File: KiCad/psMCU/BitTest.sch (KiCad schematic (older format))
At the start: 40 parts

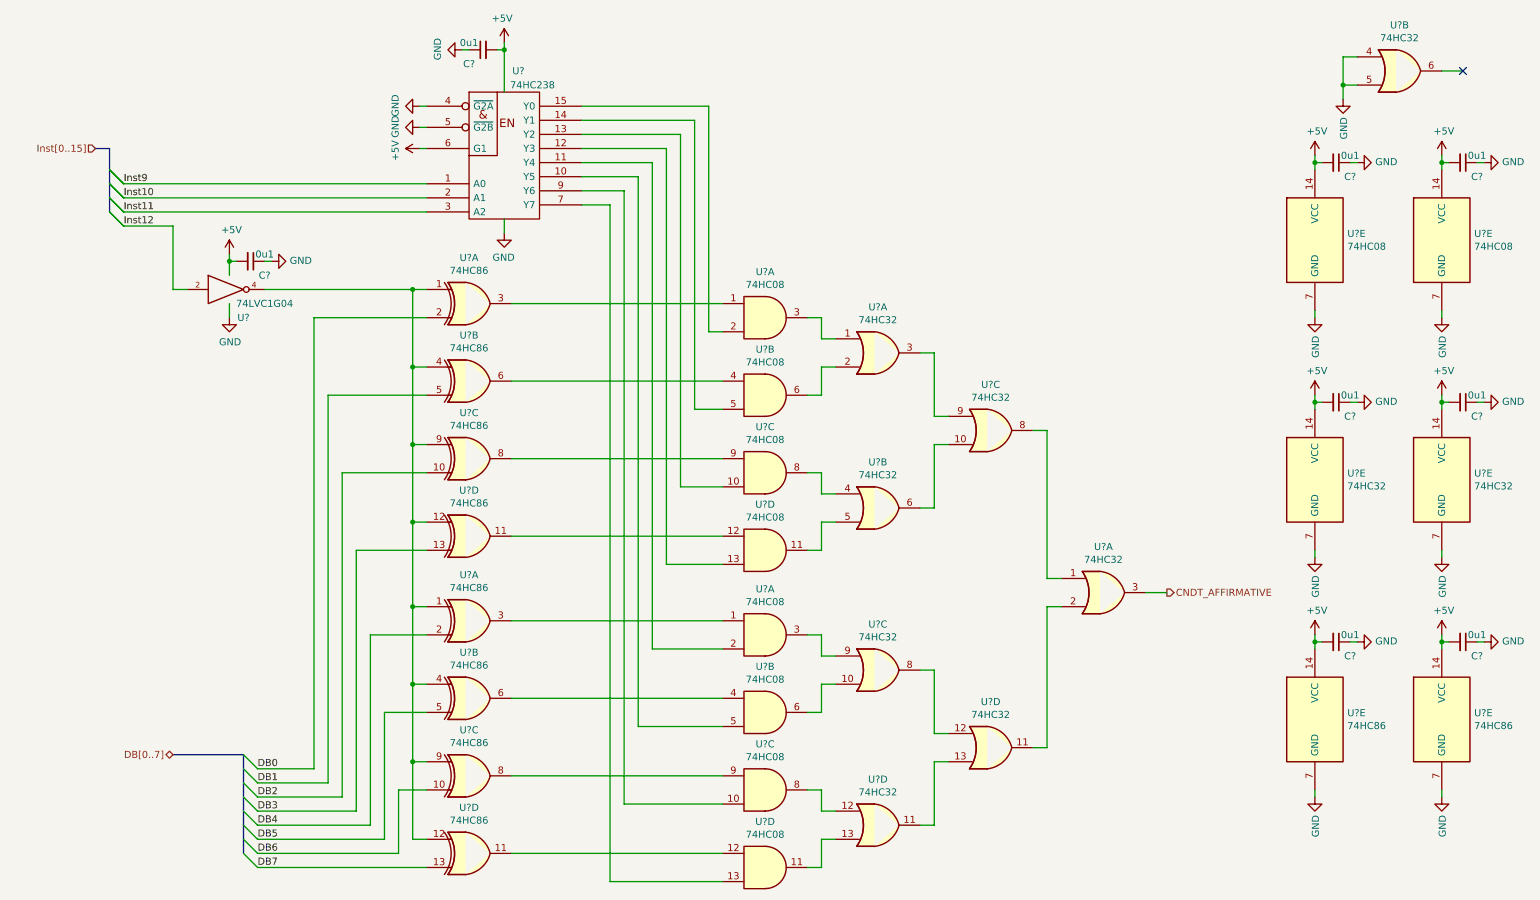
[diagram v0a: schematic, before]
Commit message: First Schematic Draft done.
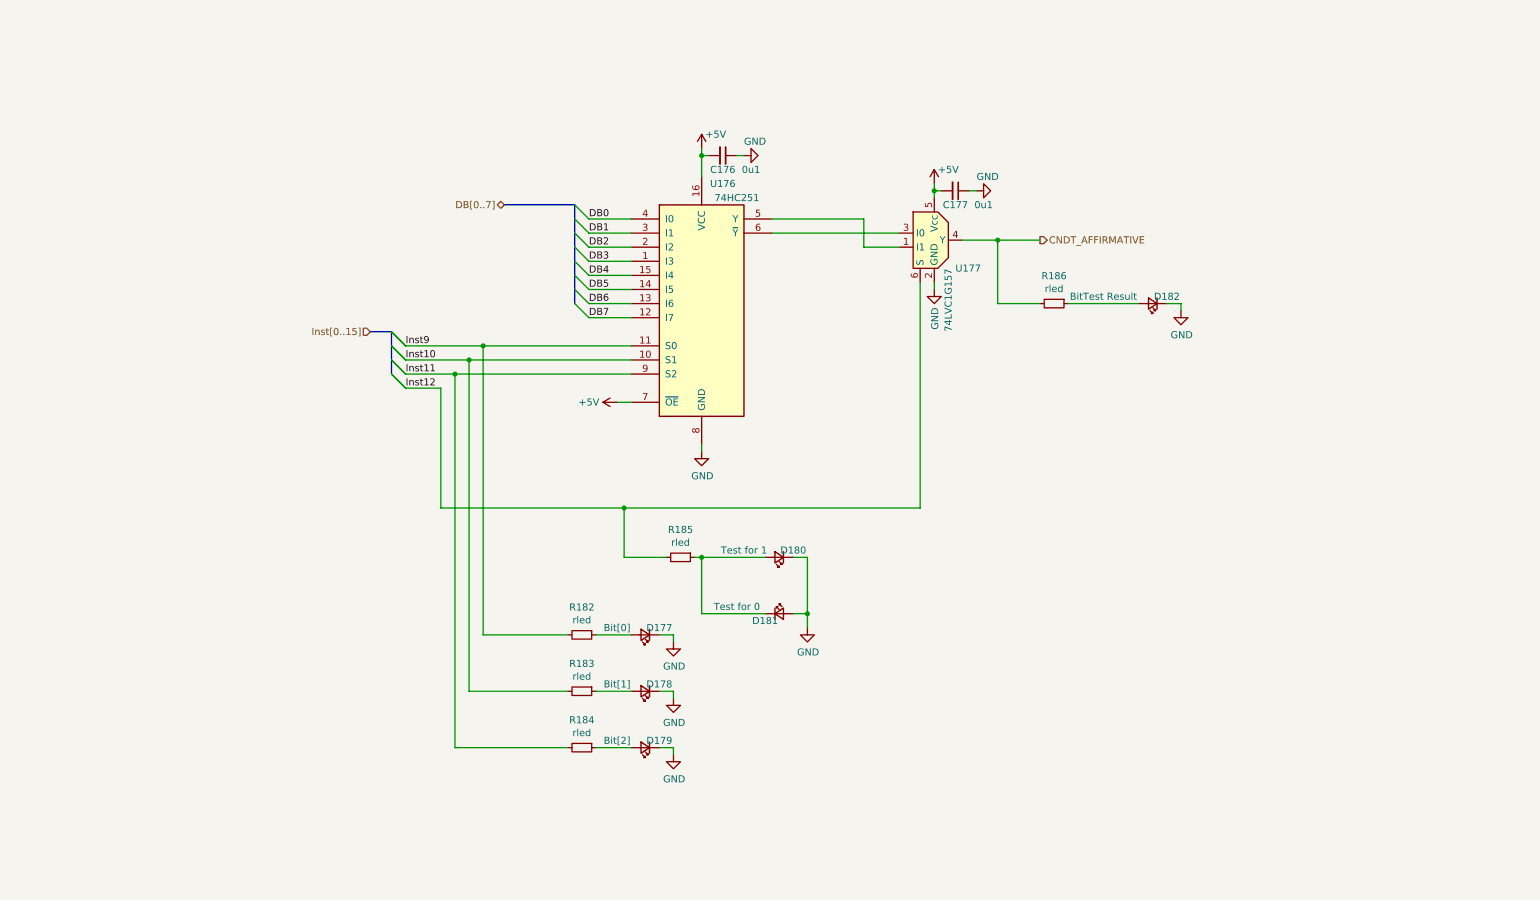
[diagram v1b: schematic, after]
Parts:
- removed C? (x8): 0u1, Capacitor_SMD:C_0603_1608Metric, symbol Device:C_Small
- removed U?: 74HC238, symbol 74xx_IEEE:74HC238
- removed U? (x10): 74HC08, symbol 74xx:74LS08
- removed U? (x10): 74HC32, symbol 74xx:74LS32
- removed U? (x10): 74HC86, symbol 74xx:74HC86
- removed U?: 74LVC1G04, Package_TO_SOT_SMD:SOT-353_SC-70-5, symbol 74xGxx:74LVC1G04
- added C176, C177: 0u1, NoRef_Footprints:C_0603_1608Metric_NoRef, symbol Device:C_Small
- added D177: Bit[0], NoRef_Footprints:D_0603_1608Metric_NoRef, symbol Device:LED_Small
- added D178: Bit[1], NoRef_Footprints:D_0603_1608Metric_NoRef, symbol Device:LED_Small
- added D179: Bit[2], NoRef_Footprints:D_0603_1608Metric_NoRef, symbol Device:LED_Small
- added D180: Test for 1, NoRef_Footprints:D_0603_1608Metric_NoRef, symbol Device:LED_Small
- added D181: Test for 0, NoRef_Footprints:D_0603_1608Metric_NoRef, symbol Device:LED_Small
- added D182: BitTest Result, NoRef_Footprints:D_0603_1608Metric_NoRef, symbol Device:LED_Small
- added R182, R183, R184, R185, R186: rled, NoRef_Footprints:R_0603_1608Metric, symbol Device:R_Small
- added U176: 74HC251, symbol 74xx:74LS251
- added U177: 74LVC1G157, Package_TO_SOT_SMD:SOT-363_SC-70-6, symbol 74LVC1G157:74LVC1G157
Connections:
- net +5V: now also C176.2, C177.2, U176.16 (VCC), U176.7 (~OE), U177.5 (Vcc)
- net CNDT_AFFIRMATIVE: now also R186.2, U177.4 (Y)
- net DB0: now also U176.4 (I0)
- net DB1: now also U176.3 (I1)
- net DB2: now also U176.2 (I2)
- net DB3: now also U176.1 (I3)
- net DB4: now also U176.15 (I4)
- net DB5: now also U176.14 (I5)
- net DB6: now also U176.13 (I6)
- net DB7: now also U176.12 (I7)
- net GND: now also C176.1, C177.1, D177.1 (K), D178.1 (K), D179.1 (K), D180.1 (K), D181.2 (A), D182.1 (K), U176.8 (GND), U177.2 (GND)
- net Inst10: now also R183.2, U176.10 (S1)
- net Inst11: now also R184.2, U176.9 (S2)
- net Inst12: now also R185.2, U177.6 (S)
- net Inst9: now also R182.2, U176.11 (S0)
- new net: U176.5 (Y), U177.1 (I1)
- new net: U176.6 (~Y), U177.3 (I0)
- new net: D182.2 (A), R186.1
- new net: D180.2 (A), D181.1 (K), R185.1
- new net: D177.2 (A), R182.1
- new net: D178.2 (A), R183.1
- new net: D179.2 (A), R184.1
- no-connect marks 1 -> 0
